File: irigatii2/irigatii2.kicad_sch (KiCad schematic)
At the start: 44 parts, among them IC1 MIC3172YN, IC2 PCA9575PW2,118, J2 Conn_01x05, T1 Transformer_1P_1S, U1 NJM2114, U2 TL431LP

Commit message: d
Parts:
- added C18, C19: 22u, Capacitor_THT:CP_Radial_D5.0mm_P2.00mm, symbol Device:C_Polarized_Small
- added C20, C21, C22: 220u, Capacitor_THT:CP_Radial_D8.0mm_P3.80mm, symbol Device:C_Small
- C1, C3, C4, C6: value C_Small -> 220u; footprint Capacitor_THT:CP_Axial_L11.0mm_D5.0mm_P18.00mm_Horizontal -> Capacitor_THT:CP_Radial_D8.0mm_P3.80mm
- C5: value C_Small -> 1u; footprint Capacitor_THT:CP_Axial_L11.0mm_D5.0mm_P18.00mm_Horizontal -> Capacitor_THT:C_Disc_D4.3mm_W1.9mm_P5.00mm
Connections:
- net +12V: now also C6.1, C18.1, C20.1, C21.1, C22.1; no longer C5.1
- net D1_1: now also IC2.12 (P0_6); no longer IC2.4 (P0_0)
- net D1_2: now also IC2.13 (P0_7); no longer IC2.5 (P0_1)
- net D2_1: now also IC2.11 (P0_5); no longer IC2.6 (P0_2)
- net D2_2: now also IC2.10 (P0_4); no longer IC2.7 (P0_3)
- net D3_1: now also IC2.4 (P0_0); no longer IC2.10 (P0_4)
- net D3_2: now also IC2.5 (P0_1); no longer IC2.11 (P0_5)
- net D3_3: now also IC2.6 (P0_2); no longer IC2.12 (P0_6)
- net D3_4: now also IC2.7 (P0_3); no longer IC2.13 (P0_7)
- net GND: now also C5.1, C6.2, C19.1, C20.2, C21.2, C22.2; no longer C5.2, C6.1
- net at C2.1, IC1.5 (VIN), R1.2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: now also C5.2; no longer C6.2
- new net: C18.2, C19.2
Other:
- moved on the sheet: C3

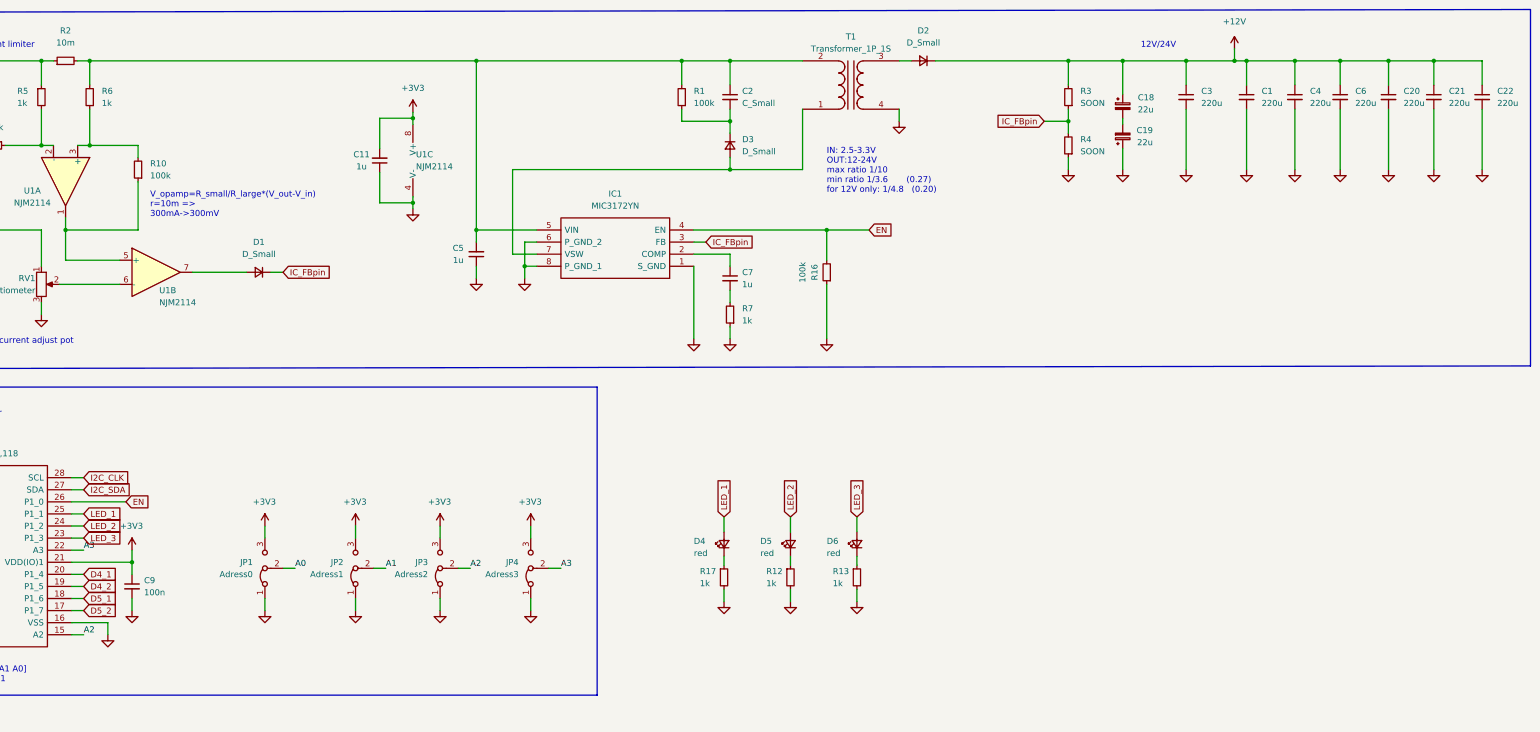
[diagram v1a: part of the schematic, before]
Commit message: v
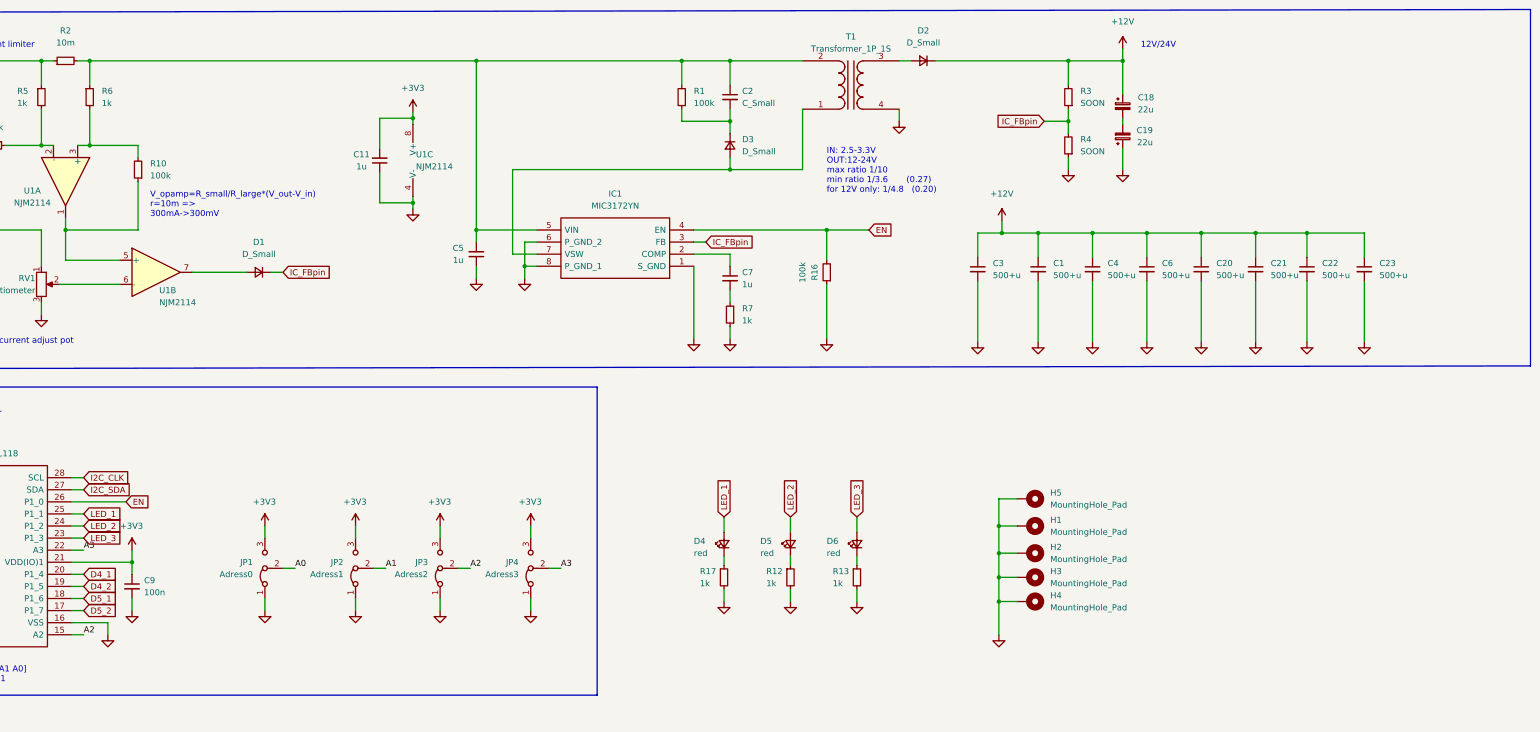
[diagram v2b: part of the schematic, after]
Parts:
- added C23: 500+u, Capacitor_THT:CP_Radial_D13.0mm_P5.00mm, symbol Device:C_Small
- added H1, H2, H3, H4, H5: MountingHole_Pad, MountingHole:MountingHole_3.2mm_M3_Pad_TopBottom, symbol Mechanical:MountingHole_Pad
- C1, C20, C21, C22, C3, C4, C6: value 220u -> 500+u; footprint Capacitor_THT:CP_Radial_D8.0mm_P3.80mm -> Capacitor_THT:CP_Radial_D13.0mm_P5.00mm
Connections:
- net +12V: now also C23.1
- net GND: now also C23.2, H1.1, H2.1, H3.1, H4.1, H5.1
- net at R10.2, U1.3 (+): now also R6.2; no longer R6.1
- net at C2.1, C5.2, IC1.5 (VIN)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: now also R6.1; no longer R6.2
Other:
- moved on the sheet: C3, R6
